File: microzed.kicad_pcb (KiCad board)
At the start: 10 copper layers, 60 x 100 mm, 333 parts, among them IC1 XC7Z020-1CLG484C, IC2 RTL8211E-VL-CG, J1 640456-3, J2 10104111-0001LF, J3 L829-1J1T-43, J4 Micro_SD_Card_Det_Hirose_DM3AT, J5 10104111-0001LF, J6 BSH-090-01-X-D-A, J7 BSH-090-01-X-D-A, Q1 MMBT3904, Q2 MMBT3904, SW1 SW_Push, U1 TLV62130RGTR, U10 MT41K256M16TW, U11 MT25QL128ABA8E12-1SIT, U12 USB3320C-EZK, U13 ASDMB-24.000MHZ-LC-T, U14 ASDMB-25.000MHZ-LC-T, U15 TXS02612RTWR, U16 CP2104-F03-GM, U2 TLV62130RGTR, U3 TLV62130RGTR, U4 TLV62130RGTR, U5 TLV62130RGTR, U6 ASDMB-33.333MHZ-LC-T, U7 TPS51206DSQR, U8 REF3012, U9 MT41K256M16TW

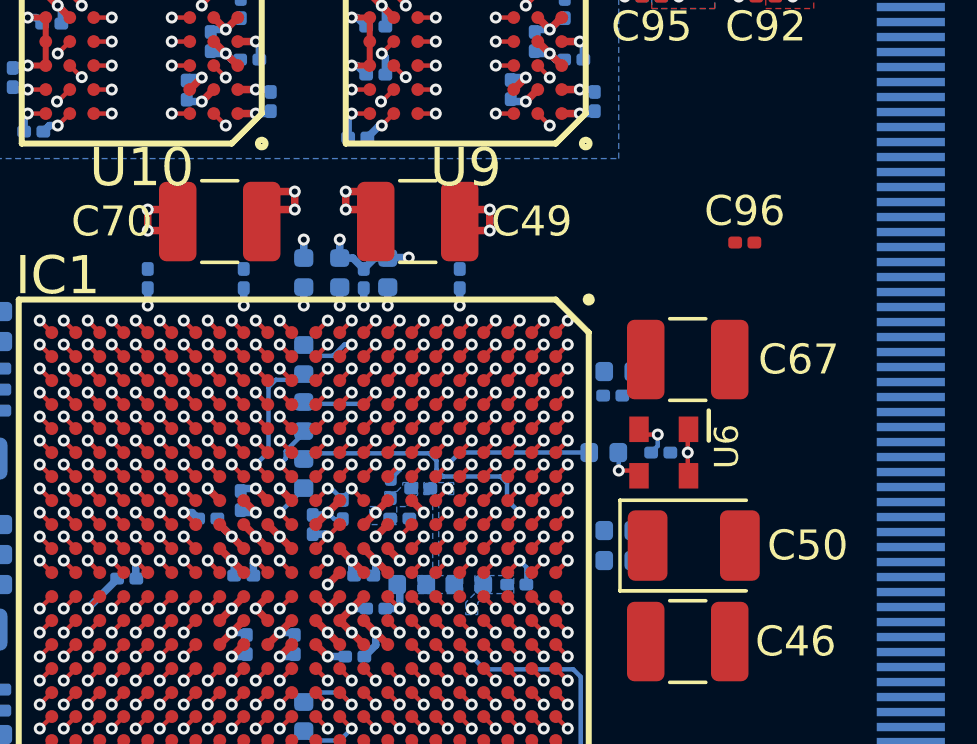
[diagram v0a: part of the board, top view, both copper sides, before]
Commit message: pcb: vttref capacitor done
Signed-off-by: Yi Qingliang <niqingliang2003@gmail.com>
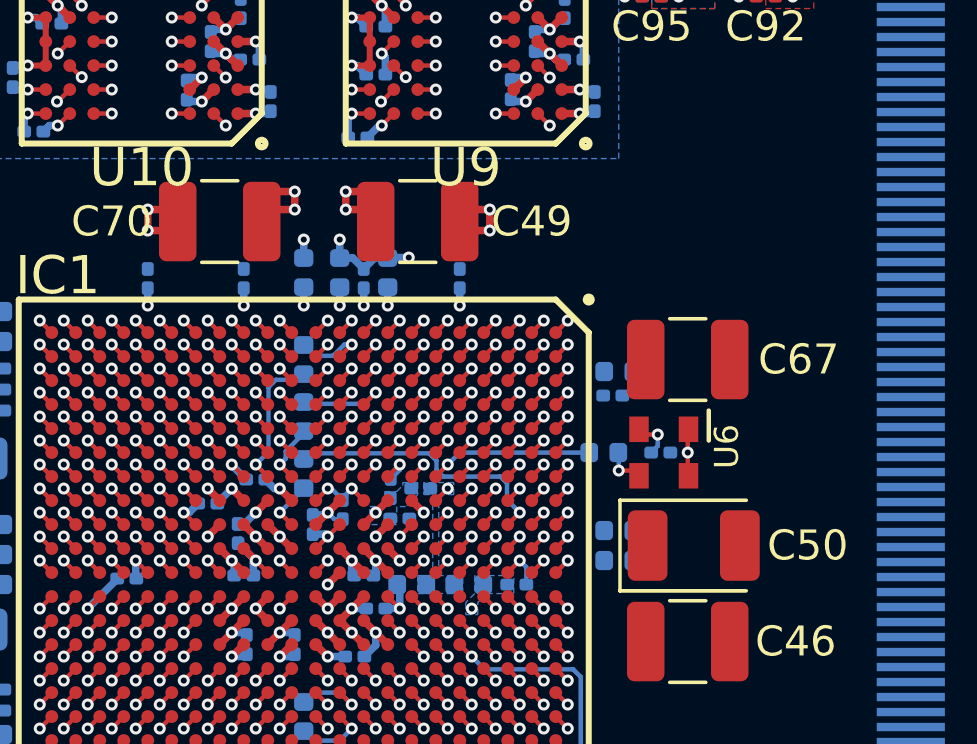
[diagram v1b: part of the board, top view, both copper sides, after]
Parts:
- C96: moved to B.Cu
- moved C96 18.1 mm to (-2.70, 47.0)
- moved C64 1.10 mm to (-3.30, 48.8)
- moved C80 0.50 mm to (-4.30, 47.8)
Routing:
- net GND: track 144.0 -> 145.0 mm
- net VTTREF: track 7.68 -> 8.38 mm
